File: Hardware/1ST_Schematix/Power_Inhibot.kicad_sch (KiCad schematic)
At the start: 2 parts, among them J1 USB_C_Receptacle_PowerOnly_24P, U2 BQ25895RTW

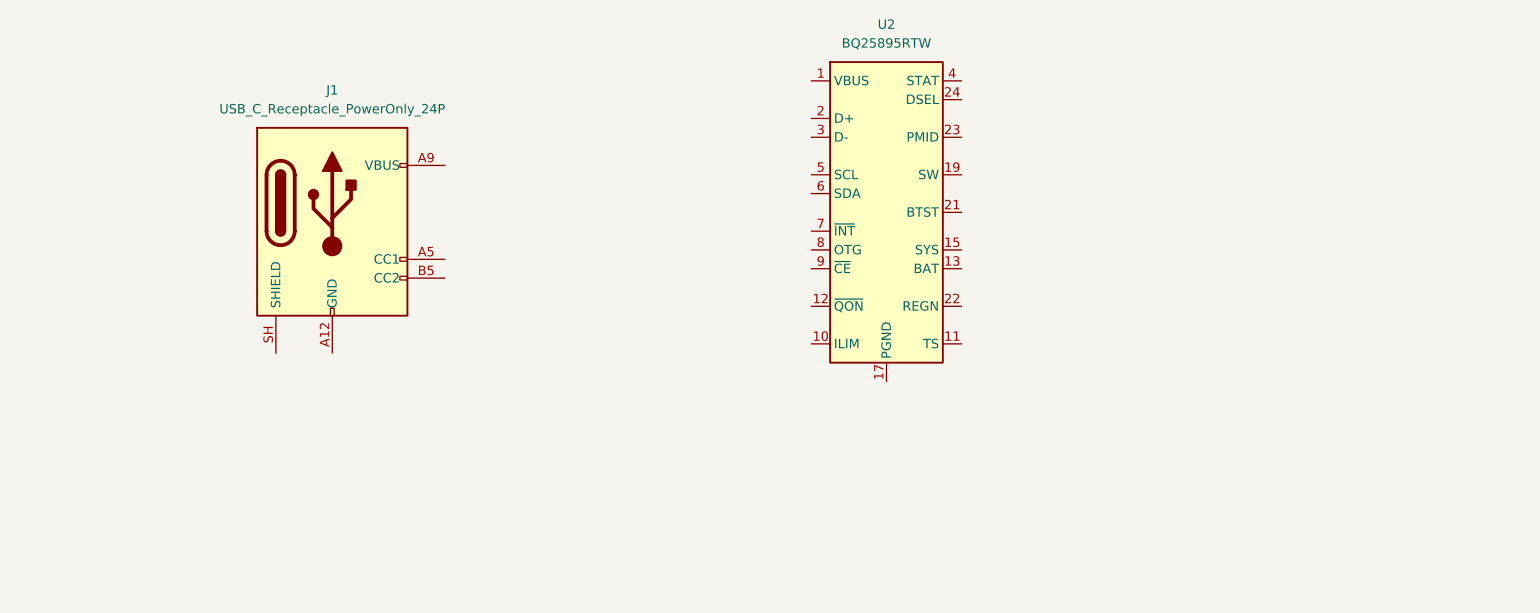
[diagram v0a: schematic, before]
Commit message: Power
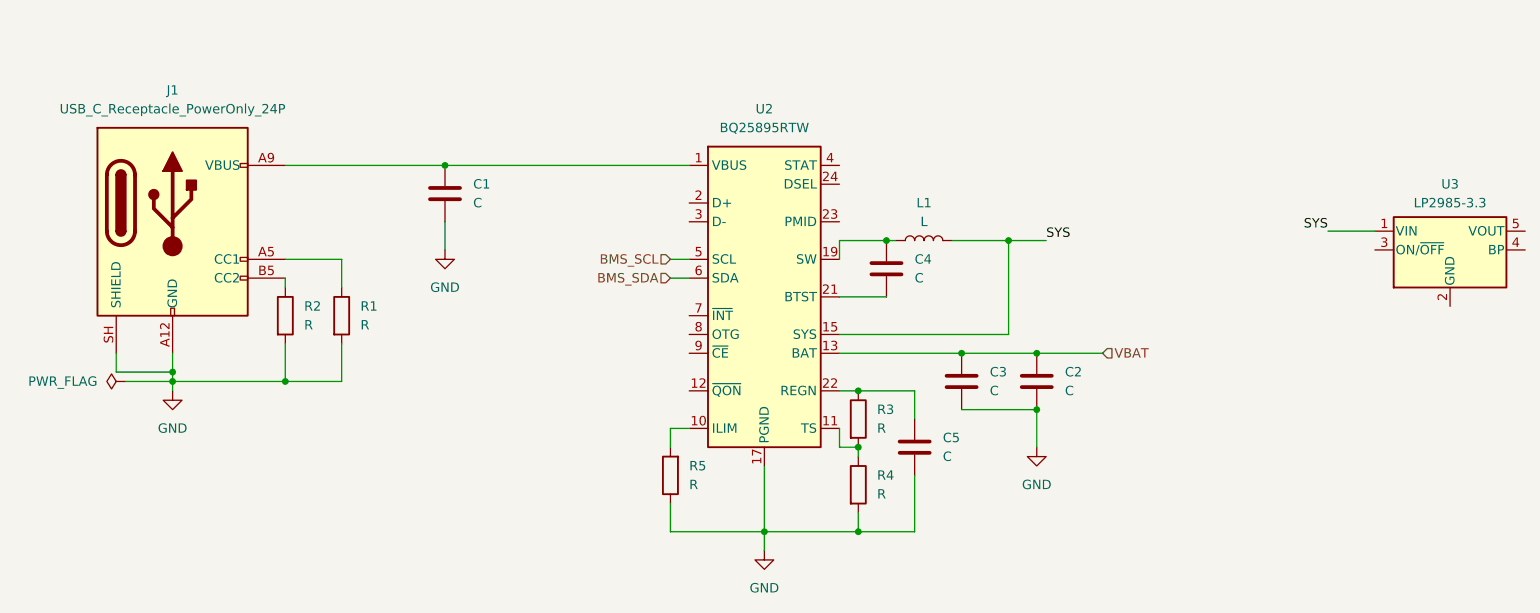
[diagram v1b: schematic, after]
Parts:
- added C1, C2, C3, C4, C5: C, symbol Device:C
- added L1: L, Package_SO:SOIC-16_3.9x9.9mm_P1.27mm, symbol Device:L
- added R1, R2, R3, R4, R5: R, symbol Device:R
- added U3: LP2985-3.3, Package_TO_SOT_SMD:SOT-23-5, symbol Regulator_Linear:LP2985-3.3
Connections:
- net GND: now reaches J1.A1 (GND), J1.A12 (GND), J1.B1 (GND), J1.B12 (GND)
- net GND: now also J1.SH (SHIELD), U2.17 (PGND), U2.18 (PGND), U2.25 (PGND), C1.2, C2.2, C3.2, C5.1, R1.2, R2.2, R4.2, R5.1
- net at J1.A4 (VBUS), J1.A9 (VBUS), J1.B4 (VBUS)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: now also U2.1 (VBUS), C1.1
- net at J1.A5 (CC1): now also R1.1
- net at J1.B5 (CC2): now also R2.1
- net at U2.10 (ILIM): now also R5.2
- net at U2.11 (TS): now also R3.2, R4.1
- net VBAT: now reaches U2.13 (BAT), U2.14 (BAT)
- net VBAT: now also C2.1, C3.1
- net SYS: now reaches U2.15 (SYS), U2.16 (SYS)
- net SYS: now also L1.2, U3.1 (VIN)
- net at U2.19 (SW), U2.20 (SW): now also C4.2, L1.1
- net at U2.21 (BTST): now also C4.1
- net at U2.22 (REGN): now also C5.2, R3.1
- net BMS_SCL: now reaches U2.5 (SCL)
- net BMS_SDA: now reaches U2.6 (SDA)
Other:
- moved on the sheet: J1, U2
